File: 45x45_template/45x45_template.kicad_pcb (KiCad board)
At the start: 2 copper layers, 45 x 45 mm, 9 parts, among them J1 Screw_Terminal_01x02

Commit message: Edge vias 0.
Merge attempt.
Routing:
- net 0: vias 0 -> 109
- net (no net): vias 109 -> 0

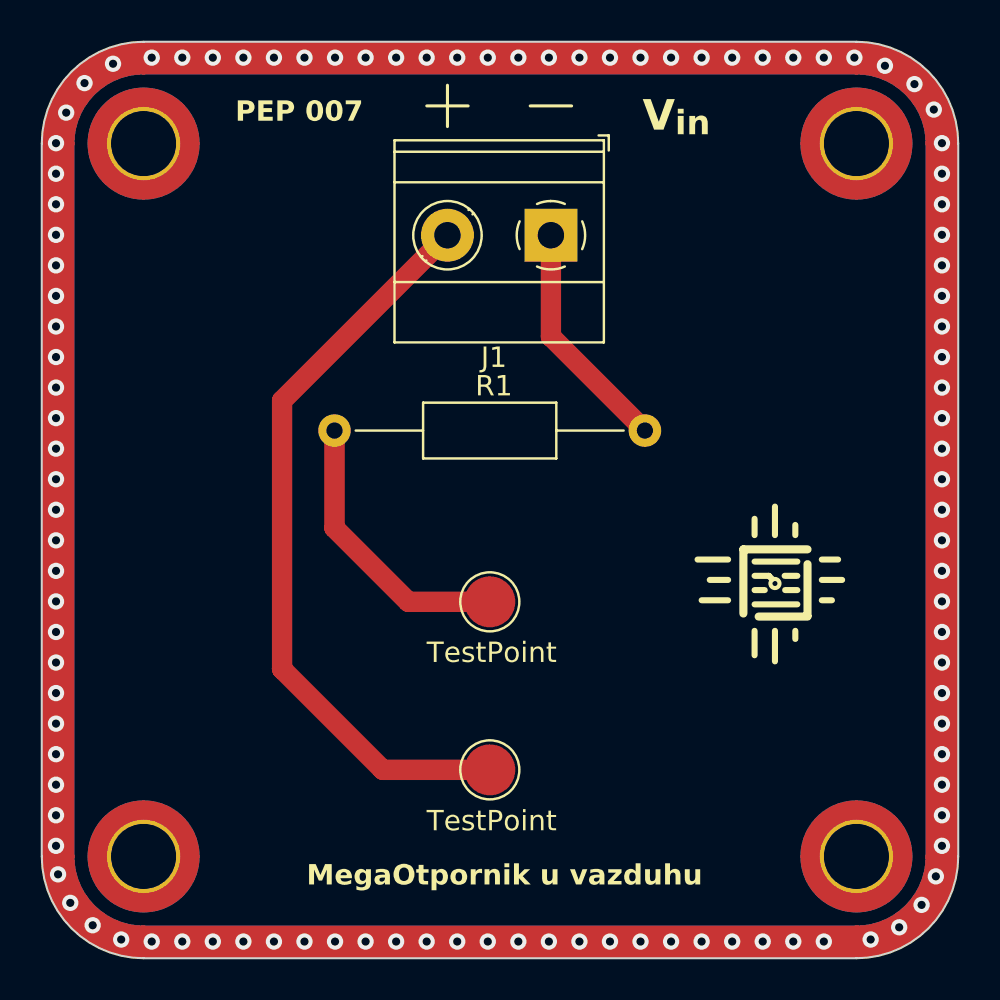
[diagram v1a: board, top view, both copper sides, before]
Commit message: Edge vias 0.
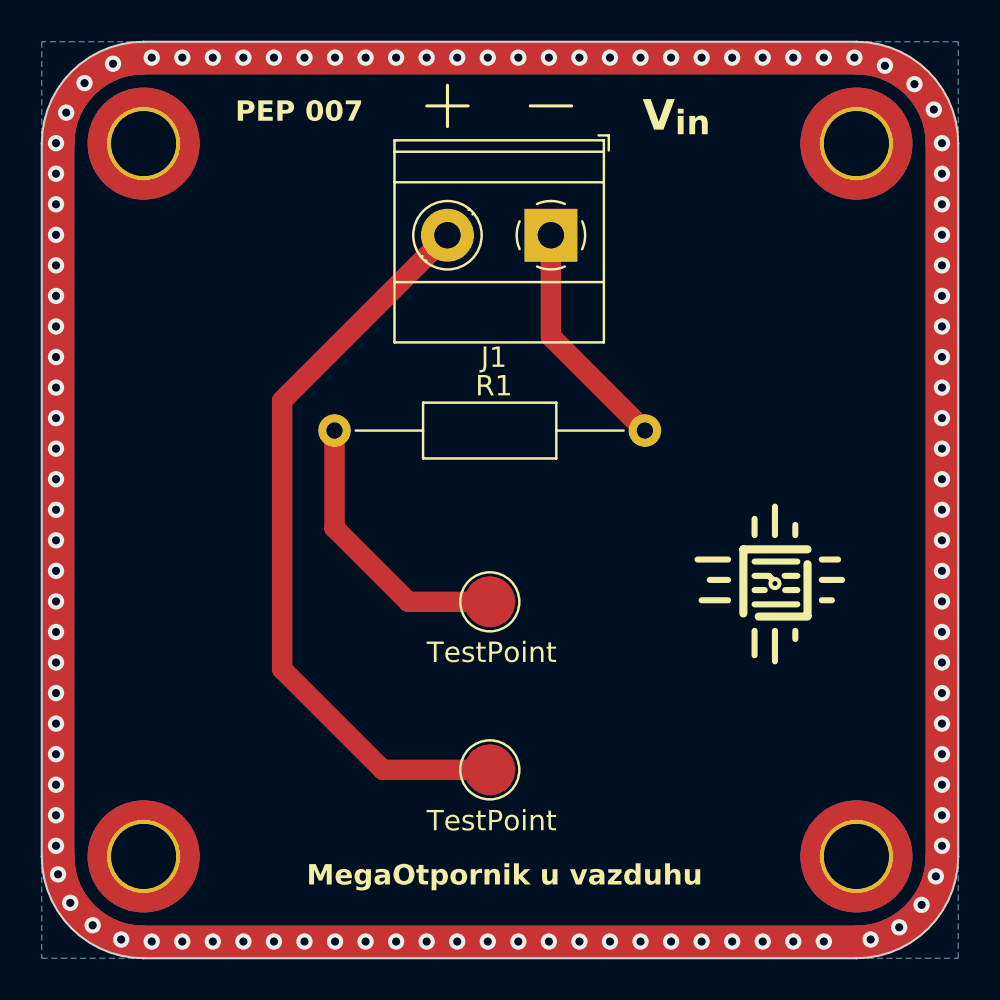
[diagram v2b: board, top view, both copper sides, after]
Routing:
- added copper zone on B.Cu, net 0
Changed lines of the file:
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@@
 		(net 3)
+	)
+	(zone
+		(net 1)
+		(net_name "0")
+		(layer "B.Cu")
+		(hatch edge 0.5)
+		(connect_pads
+			(clearance 0.5)
+		)
+		(min_thickness 0.25)
+		(filled_areas_thickness no)
+		(fill yes
+			(thermal_gap 0.5)
+			(thermal_bridge_width 0.5)
+		)
+		(polygon
+			(pts
+				(xy 100 100) (xy 100 145) (xy 145 145) (xy 145 100)
+			)
+		)
 	)
 	(embedded_fonts no)
